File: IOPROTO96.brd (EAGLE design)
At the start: 38.1 x 39.4 mm, 5 parts

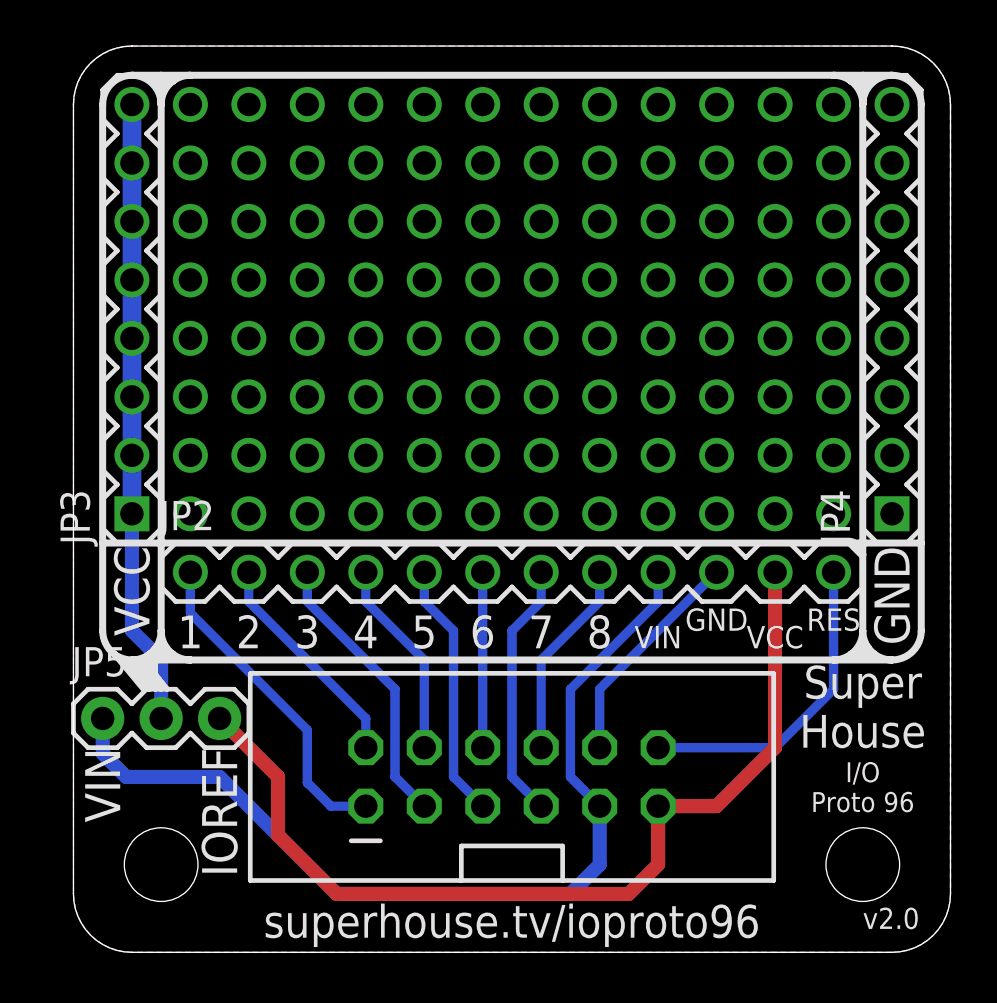
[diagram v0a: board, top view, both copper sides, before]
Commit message: Final routing and DRC for release v2.0
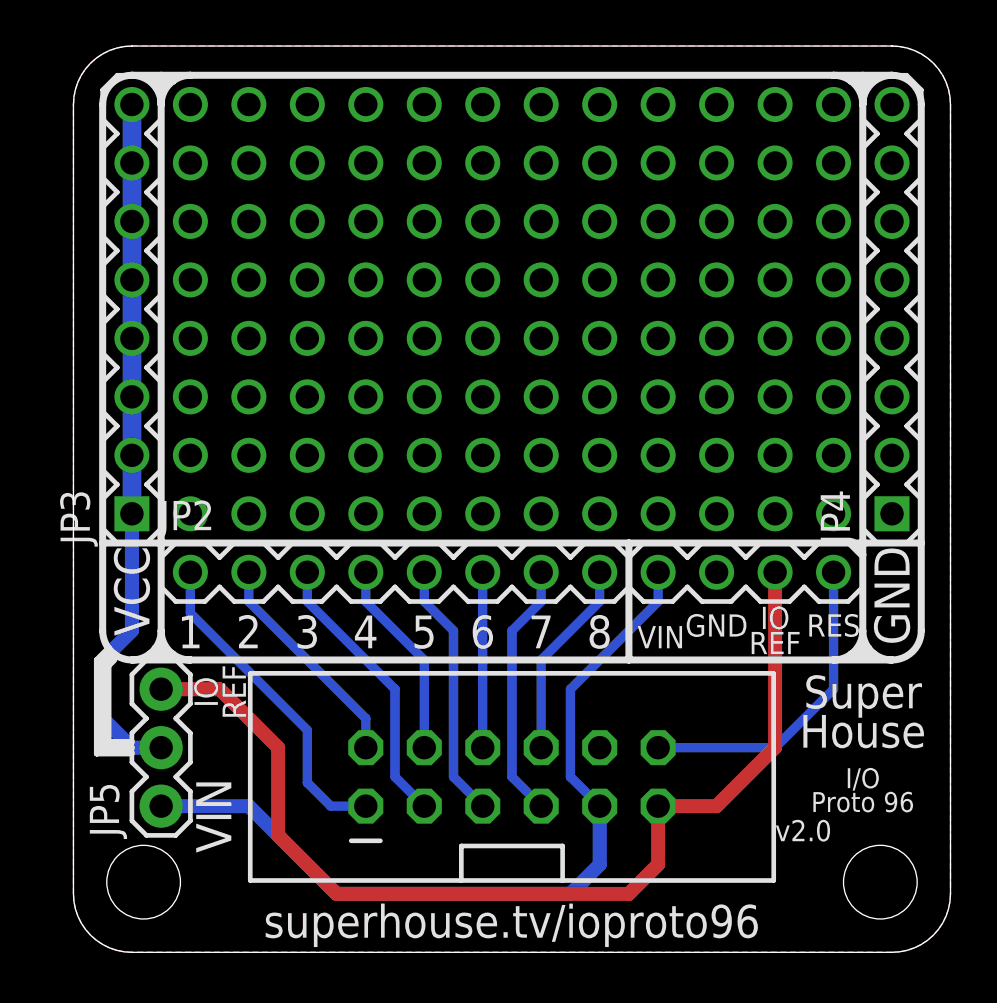
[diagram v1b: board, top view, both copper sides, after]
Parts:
- moved JP5 4.58 mm to (3.81, 6.35), turned to 90 degrees
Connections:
- net D1 renamed IO1
- net D2 renamed IO2
- net D3 renamed IO3
- net D4 renamed IO4
- net D5 renamed IO5
- net D6 renamed IO6
- net D7 renamed IO7
- net D8 renamed IO8
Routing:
- net GND: track 9.72 -> 0.00 mm
- net VIN: track 41.0 -> 36.0 mm
- net IOREF: track 40.5 -> 44.3 mm
- net V+: track 27.2 -> 30.3 mm
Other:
- board text added: "IO REF"
